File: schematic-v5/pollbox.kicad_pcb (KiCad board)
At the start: 2 copper layers, 49.5 x 72.4 mm, 24 parts, among them P1 CONN_01X15, P10 CONN_01X04, P2 CONN_02X03, P20 CONN_01X04, P3 CONN_01X15, P30 CONN_01X04, P40 CONN_01X04, P50 CONN_01X04, U1 NodeMCU_1.0, U2 ULN2803

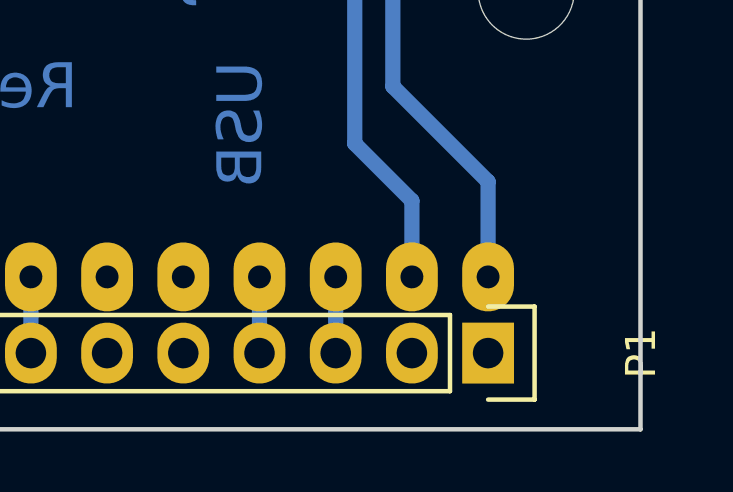
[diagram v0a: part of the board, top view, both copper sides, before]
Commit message: add missing wires
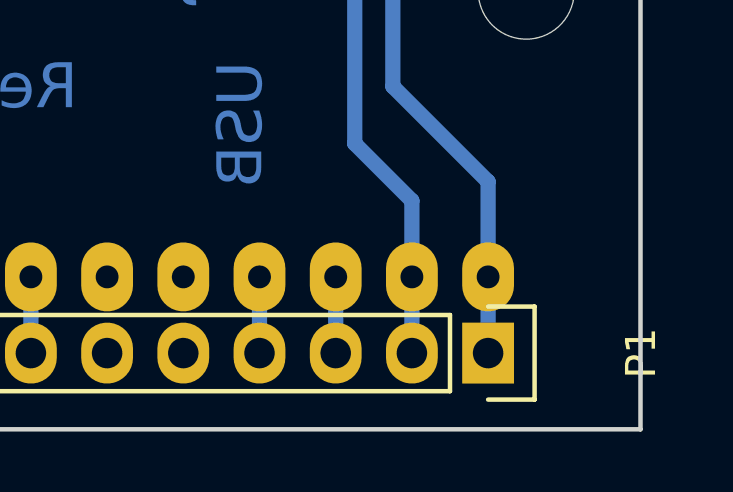
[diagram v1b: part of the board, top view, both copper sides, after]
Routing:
- net GND: track 188.7 -> 191.2 mm
- net +5V: track 106.9 -> 109.4 mm
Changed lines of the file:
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@@
-(kicad_pcb (version 4) (host pcbnew 4.0.2+dfsg1-stable)
+(kicad_pcb (version 4) (host pcbnew 4.0.3-stable)
   (general
     (links 77)
-    (no_connects 2)
-    (area 77.394999 43.739999 127.075001 118.820001)
+    (no_connects 0)
+    (area 65.810001 40.48 132.801143 121.927333)
     (thickness 1.6)
     (drawings 9)
-    (tracks 279)
+    (tracks 281)
     (zones 0)
     (modules 24)
@@
   (segment (start 118.11 66) (end 117.435 66) (width 0.3048) (layer B.Cu) (net 1) (status 30))
   (segment (start 121.92 90.805) (end 121.92 90.805) (width 0.508) (layer B.Cu) (net 1) (status 30))
+  (segment (start 121.92 114.3) (end 121.92 116.84) (width 0.508) (layer B.Cu) (net 2))
   (segment (start 121.92 114.3) (end 121.92 111.125) (width 0.508) (layer B.Cu) (net 2))
   (segment (start 121.92 111.125) (end 118.745 107.95) (width 0.508) (layer B.Cu) (net 2))
@@
   (segment (start 106.68 57.785) (end 114.3 57.785) (width 0.508) (layer B.Cu) (net 2) (status 30))
   (segment (start 99.06 57.785) (end 106.68 57.785) (width 0.508) (layer B.Cu) (net 2) (status 10))
+  (segment (start 119.38 114.3) (end 119.38 116.84) (width 0.508) (layer B.Cu) (net 3))
   (segment (start 119.38 114.3) (end 119.38 111.76) (width 0.508) (layer B.Cu) (net 3))
   (segment (start 119.38 111.76) (end 117.475 109.855) (width 0.508) (layer B.Cu) (net 3))
@@
     (polygon
       (pts
-        (xy 127 119.38) (xy 77.47 119.38) (xy 77.47 46.99) (xy 127 46.99) (xy 127 119.38)
+        (xy 127 119.38) (xy 77.47 119.38) (xy 77.47 46.99) (xy 127 46.99)
       )
     )
